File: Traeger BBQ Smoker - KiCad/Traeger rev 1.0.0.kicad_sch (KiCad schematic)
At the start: 45 parts, among them J2 Time of Flight Sensor, J3 To Wiring Harness, J4 Spare GPIO's, J5 Rotary Encoder, J6 ADS1115 0x49, J7 Temp Sensors, J8 Temp Sensors, K1 Fan Relay, K3 Auger 1 Relay, K6 Igniter 1 Relay, Q1 BC547, Q2 BC547, Q6 BC547, U1 mini_esp32

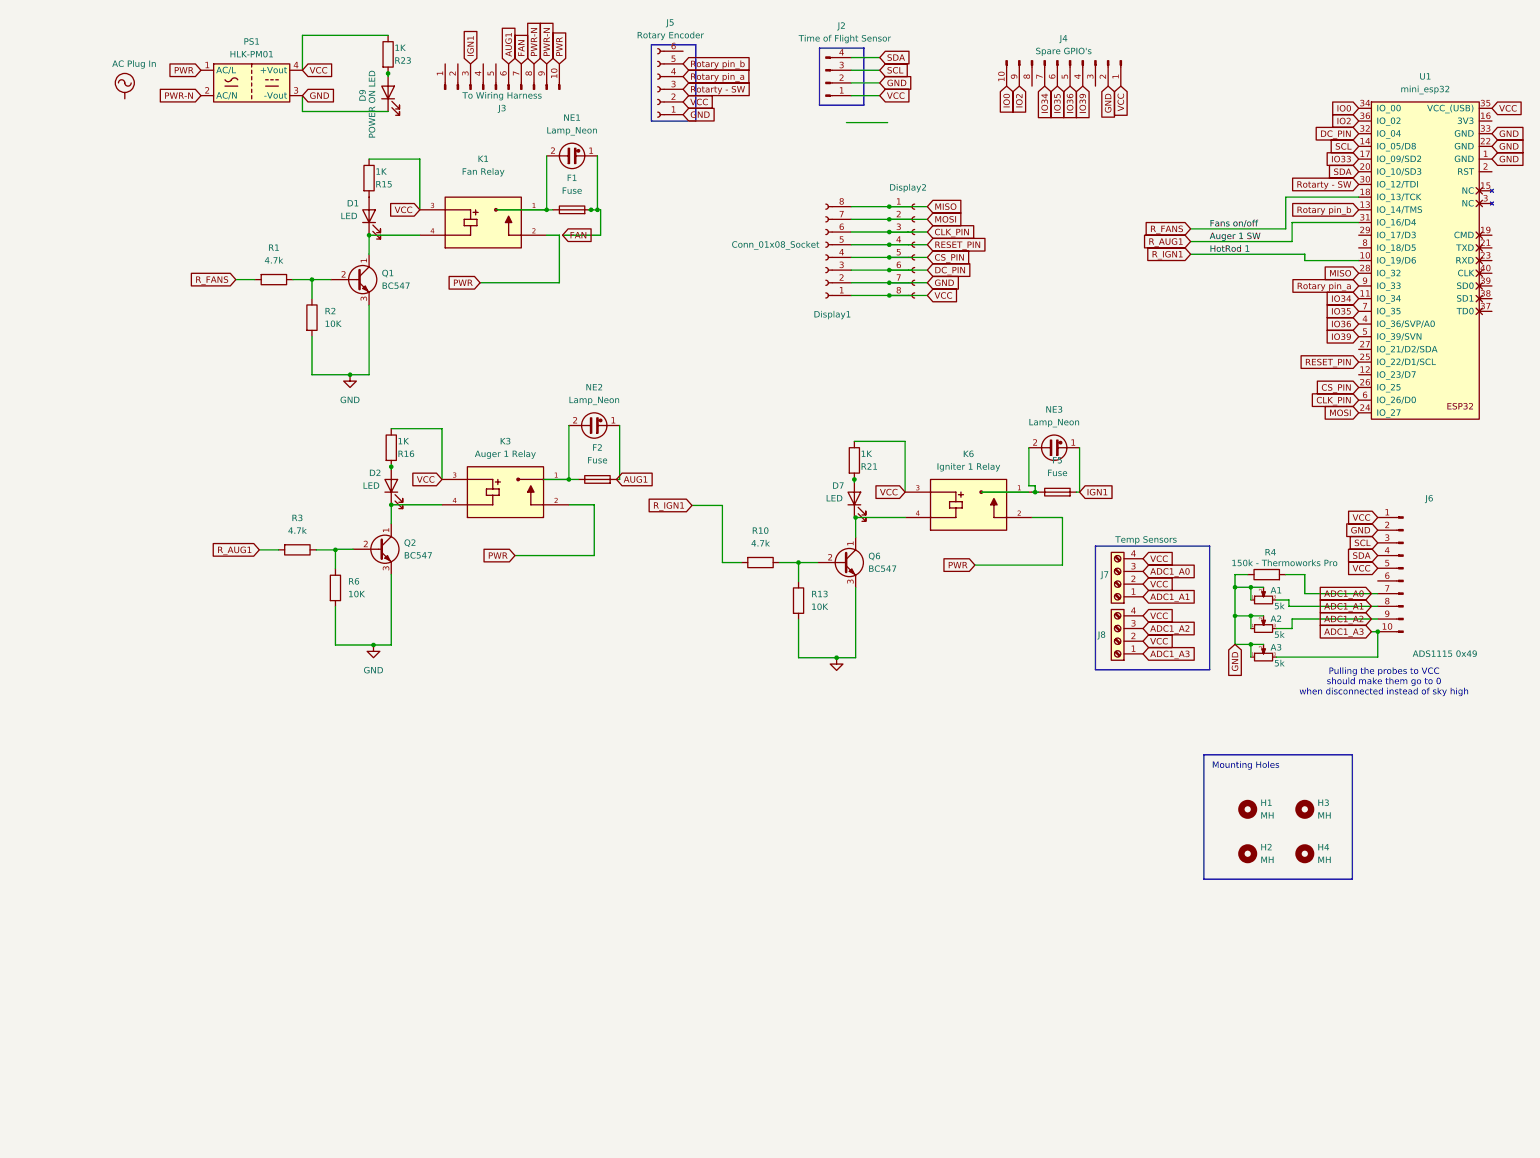
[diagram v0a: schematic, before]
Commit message: Update Traeger rev 1.0.0.kicad_sch
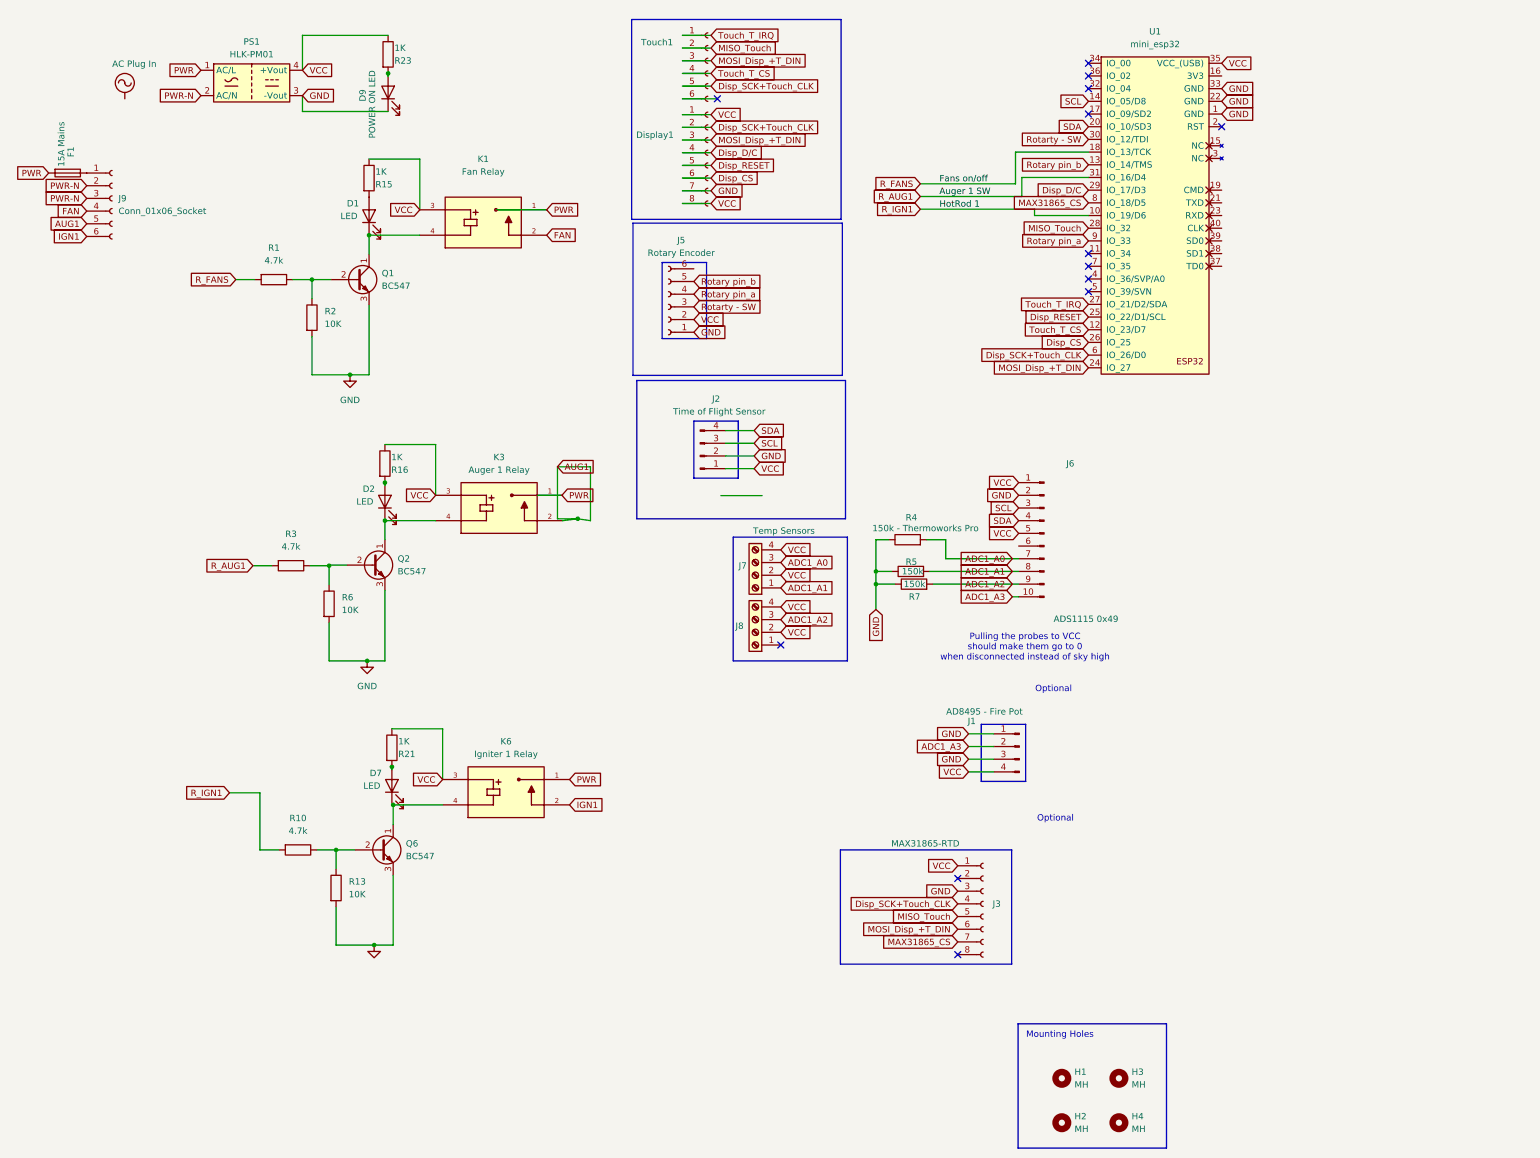
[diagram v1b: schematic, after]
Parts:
- removed A1, A2, A3: 5k, Potentiometer_THT:Potentiometer_Bourns_3296W_Vertical, symbol Device:R_Potentiometer_Small
- removed Display2: Conn_01x08_Socket, Connector_JST:JST_ZH_B8B-ZR_1x08_P1.50mm_Vertical, symbol Connector:Conn_01x08_Socket
- removed F2, F5: Fuse, Fuse:Fuse_Littelfuse_395Series, symbol Device:Fuse
- removed J3: To Wiring Harness, TerminalBlock_RND:TerminalBlock_RND_205-00010_1x10_P5.00mm_Horizontal, symbol Connector:Conn_01x10_Pin
- removed J4: Spare GPIO's, Connector_PinHeader_2.54mm:PinHeader_1x10_P2.54mm_Vertical, symbol Connector:Conn_01x10_Pin
- removed NE1, NE2, NE3: Lamp_Neon, LED_THT:LED_D3.0mm, symbol Device:Lamp_Neon
- added J1: AD8495 - Fire Pot, Connector_JST:JST_EH_B4B-EH-A_1x04_P2.50mm_Vertical, symbol Connector:Conn_01x04_Pin
- added J3: MAX31865-RTD, Connector_PinSocket_2.54mm:PinSocket_1x08_P2.54mm_Vertical, symbol Connector:Conn_01x08_Socket
- added J9: Conn_01x06_Socket, TerminalBlock_RND:TerminalBlock_RND_205-00005_1x06_P5.00mm_Horizontal, symbol Connector:Conn_01x06_Socket
- added R5, R7: 150k, Resistor_THT:R_Axial_DIN0207_L6.3mm_D2.5mm_P7.62mm_Horizontal, symbol Device:R
- added Touch1: Conn_01x06_Socket, Connector_JST:JST_EH_B6B-EH-A_1x06_P2.50mm_Vertical, symbol Connector:Conn_01x06_Socket
- Display1: footprint Connector_JST:JST_ZH_B8B-ZR_1x08_P1.50mm_Vertical -> Connector_JST:JST_EH_B8B-EH-A_1x08_P2.50mm_Vertical
- F1: value Fuse -> 15A Mains; footprint Fuse:Fuse_Littelfuse_395Series -> Fuse:Fuse Block 3544-2_KEYSTONE
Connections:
- net ADC1_A1: now also R5.2
- net ADC1_A2: now also R7.2
- net ADC1_A3: now also J1.2 (Pin_2); no longer J8.1 (Pin_1)
- net AUG1: now also K3.2, J9.5 (Pin_5)
- net FAN: now also K1.2, J9.4 (Pin_4); no longer F1.2
- net GND: now also Display1.7 (Pin_7), J1.1 (Pin_1), J1.3 (Pin_3), J3.3 (Pin_3), R5.1, R7.1; no longer Display1.2 (Pin_2)
- net IGN1: now also K6.2, J9.6 (Pin_6)
- net PWR: now also F1.2, K1.1, K3.1, K6.1; no longer K1.2, K3.2, K6.2
- net PWR-N: now also J9.2 (Pin_2), J9.3 (Pin_3)
- net VCC: now also Display1.8 (Pin_8), J1.4 (Pin_4), J3.1 (Pin_1)
- net Touch_T_CS: now reaches U1.12 (IO_23/D7)
- net Touch_T_CS: now also Touch1.4 (Pin_4)
- net Touch_T_IRQ: now reaches U1.27 (IO_21/D2/SDA)
- net Touch_T_IRQ: now also Touch1.1 (Pin_1)
- net Disp_D/C: now reaches U1.29 (IO_17/D3)
- net Disp_D/C: now also Display1.4 (Pin_4)
- net MAX31865_CS: now reaches U1.8 (IO_18/D5)
- net MAX31865_CS: now also J3.7 (Pin_7)
- net at F1.1: now also J9.1 (Pin_1); no longer K1.1
- net CLK_PIN renamed Disp_CS
- net Disp_CS: now also U1.26 (IO_25); no longer U1.6 (IO_26/D0)
- removed net CS_PIN: Display1.4 (Pin_4), U1.26 (IO_25)
- net DC_PIN: no longer names the net of U1.32 (IO_04)
- net DC_PIN: no longer Display1.3 (Pin_3)
- net IO0: no longer names the net of U1.34 (IO_00)
- net IO2: no longer names the net of U1.36 (IO_02)
- net IO33: no longer names the net of U1.17 (IO_09/SD2)
- net IO34: no longer names the net of U1.11 (IO_34)
- net IO35: no longer names the net of U1.7 (IO_35)
- net IO36: no longer names the net of U1.4 (IO_36/SVP/A0)
- net IO39: no longer names the net of U1.5 (IO_39/SVN)
- net MISO renamed MISO_Touch
- net MISO_Touch: now also J3.5 (Pin_5), Touch1.2 (Pin_2); no longer Display1.8 (Pin_8)
- net MOSI renamed MOSI_Disp_+T_DIN
- net MOSI_Disp_+T_DIN: now also Display1.3 (Pin_3), J3.6 (Pin_6), Touch1.3 (Pin_3); no longer Display1.7 (Pin_7)
- net RESET_PIN renamed Disp_RESET
- new net Disp_SCK+Touch_CLK: Display1.2 (Pin_2), J3.4 (Pin_4), Touch1.5 (Pin_5), U1.6 (IO_26/D0)
- no-connect marks 0 -> 13
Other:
- note added: "Optional"
- moved on the sheet: D2, D7, H1, H2, H3, H4, J2, J5, J6, J7, J8, K3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
